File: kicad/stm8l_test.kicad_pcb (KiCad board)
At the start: 2 copper layers, 72 x 72 mm, 60 parts, among them J1 Conn_01x04, Q1 SI2365EDS-T1-GE3, Q2 2N7002, Q3 SI2365EDS-T1-GE3, Q4 SI2365EDS-T1-GE3, Q5 SI2365EDS-T1-GE3, Q6 SI2365EDS-T1-GE3, Q7 SI2365EDS-T1-GE3, Q8 SI2365EDS-T1-GE3, SW1 prog_sw, SW2 SW_Push, SW3 Rotary_Encoder_Switch, U1 BD70522GUL-E2, U2 STM8L101F3P

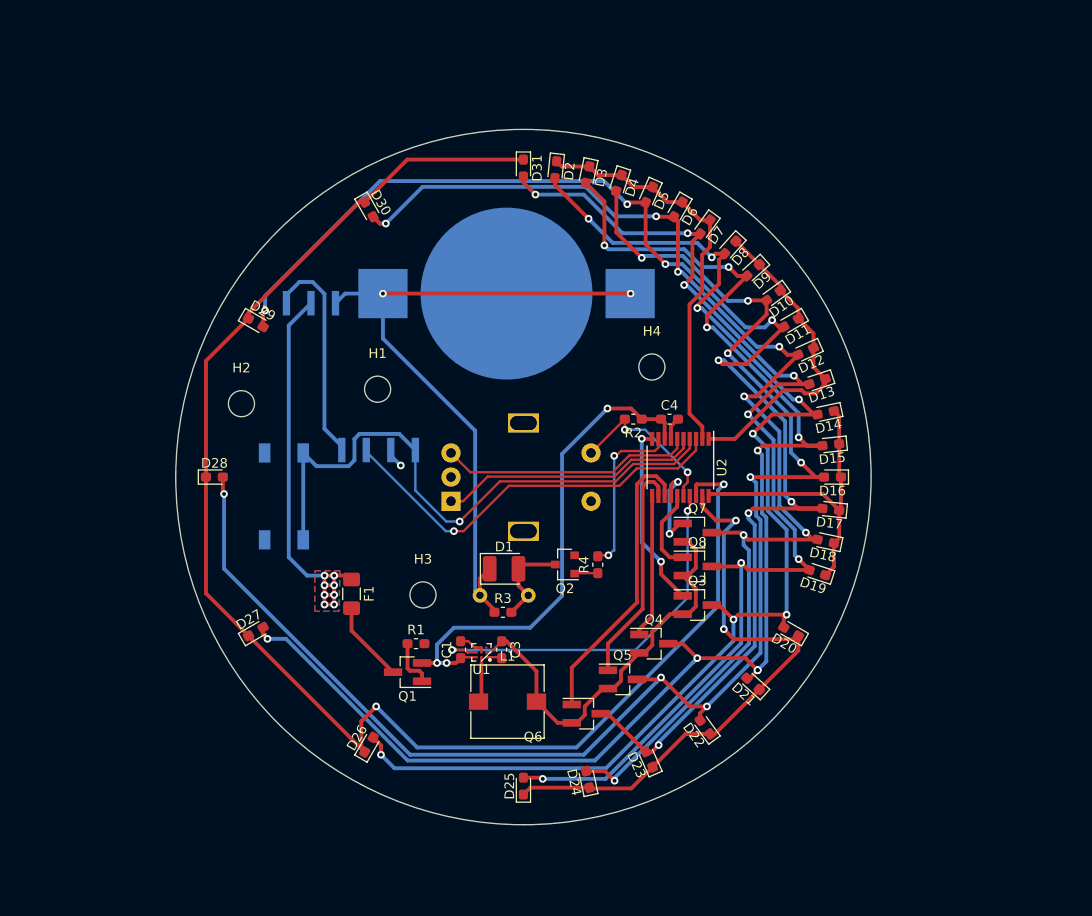
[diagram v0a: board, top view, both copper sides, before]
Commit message: PCB rev1 ordered
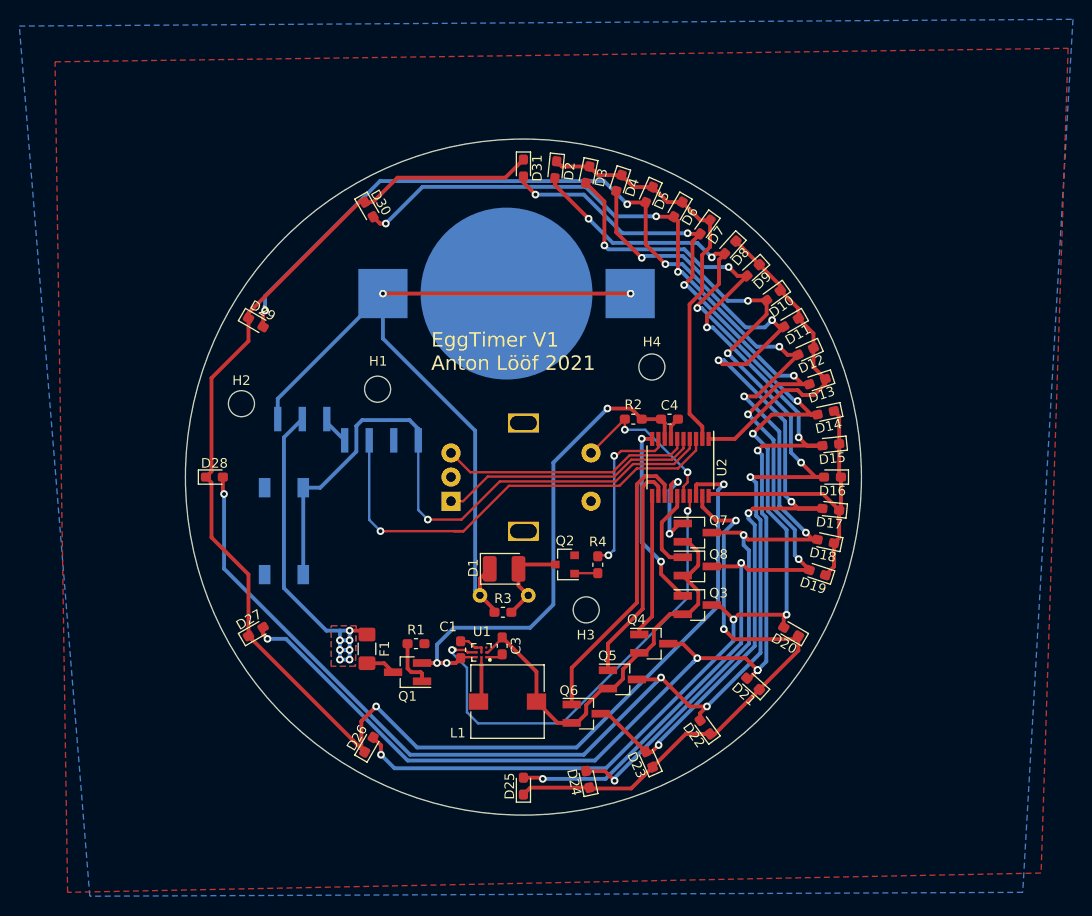
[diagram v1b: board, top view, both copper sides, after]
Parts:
- moved H3 17.0 mm to (170.3, 110.2)
- moved SW1 6.47 mm to (140.9, 87.7), turned to 180 degrees
- moved F1 5.92 mm to (147.6, 114.3)
- moved SW2 3.60 mm to (139.0, 102.1)
- moved J1 1.04 mm to (149.1, 92.7)
- moved C3 0.40 mm to (161.6, 114.0)
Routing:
- net prog_v: track 22.8 -> 2.97 mm
- net vbat: track 72.0 -> 84.2 mm
- net led_enable: track 39.9 -> 49.1 mm
- net pa0: track 42.4 -> 48.2 mm
- net Net-(F1-Pad1): track 43.7 -> 37.9 mm, vias 8 -> 7
- net Net-(F1-Pad2): track 8.41 -> 3.41 mm
- net rst: track 62.6 -> 66.7 mm
- net vcc: track 52.4 -> 55.9 mm
- net GND: track 8.94 -> 6.91 mm, vias 1 -> 0
- net vled: track 43.5 -> 44.2 mm
- added copper zone on B.Cu, net GND
- added copper zone on F.Cu, net GND
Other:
- board size 72 x 72 mm -> 70 x 70 mm
- rule pad_to_mask_clearance: 0.051 -> 0
- board text added: "3v3 pa0 gnd rst"
- board text added: "EggTimer V1 Anton Lööf 2021"
- board text added: "JLCJLCJLCJLC"
- board text added: "bat + prog"
